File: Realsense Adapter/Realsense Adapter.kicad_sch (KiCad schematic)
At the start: 2 parts, among them J1 USB3_B_Micro

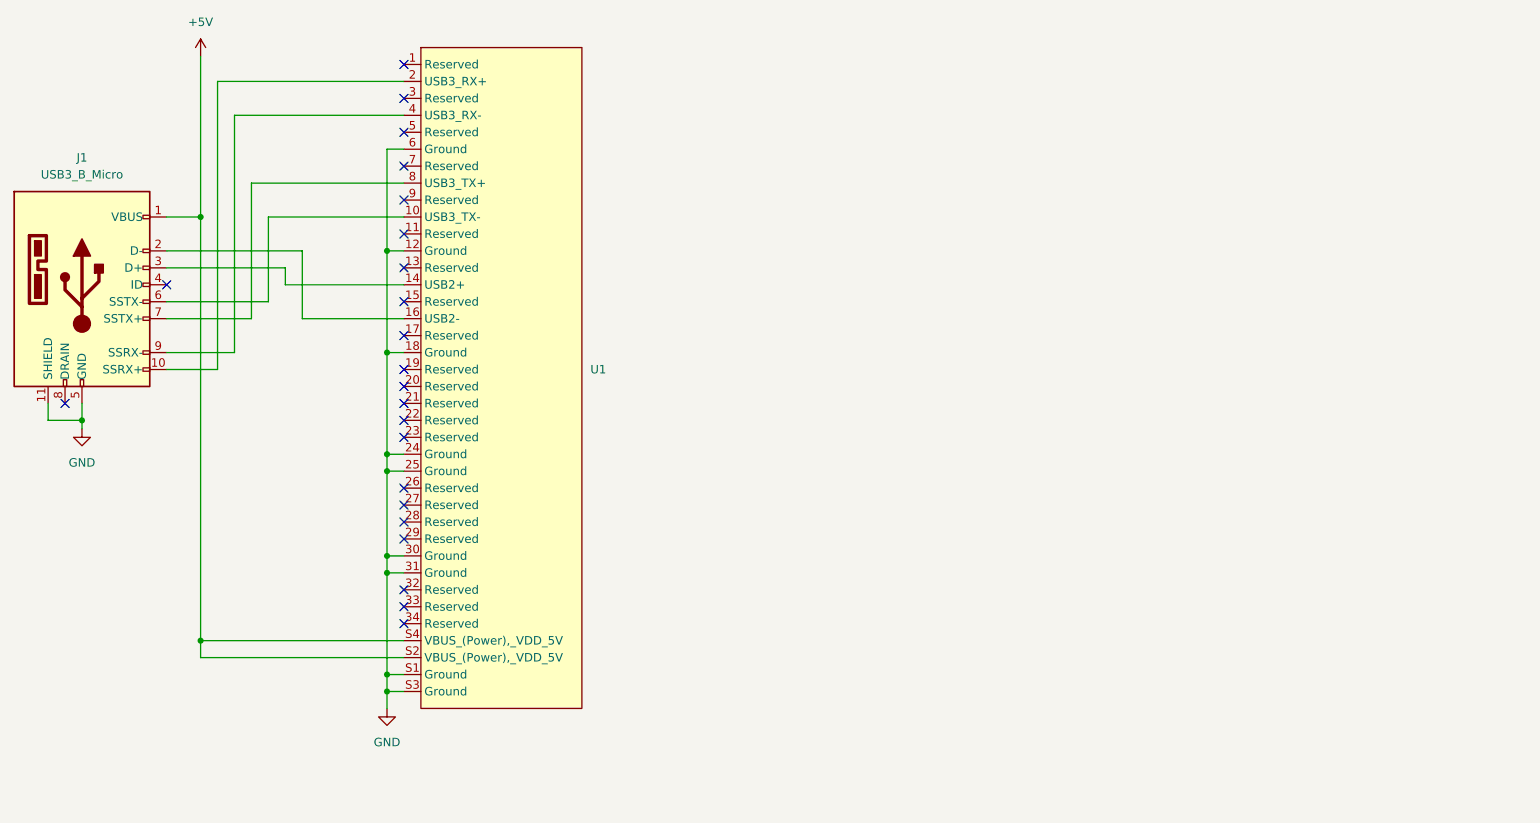
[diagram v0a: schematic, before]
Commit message: Version v1.0-PROTO of Realsense adapter complete
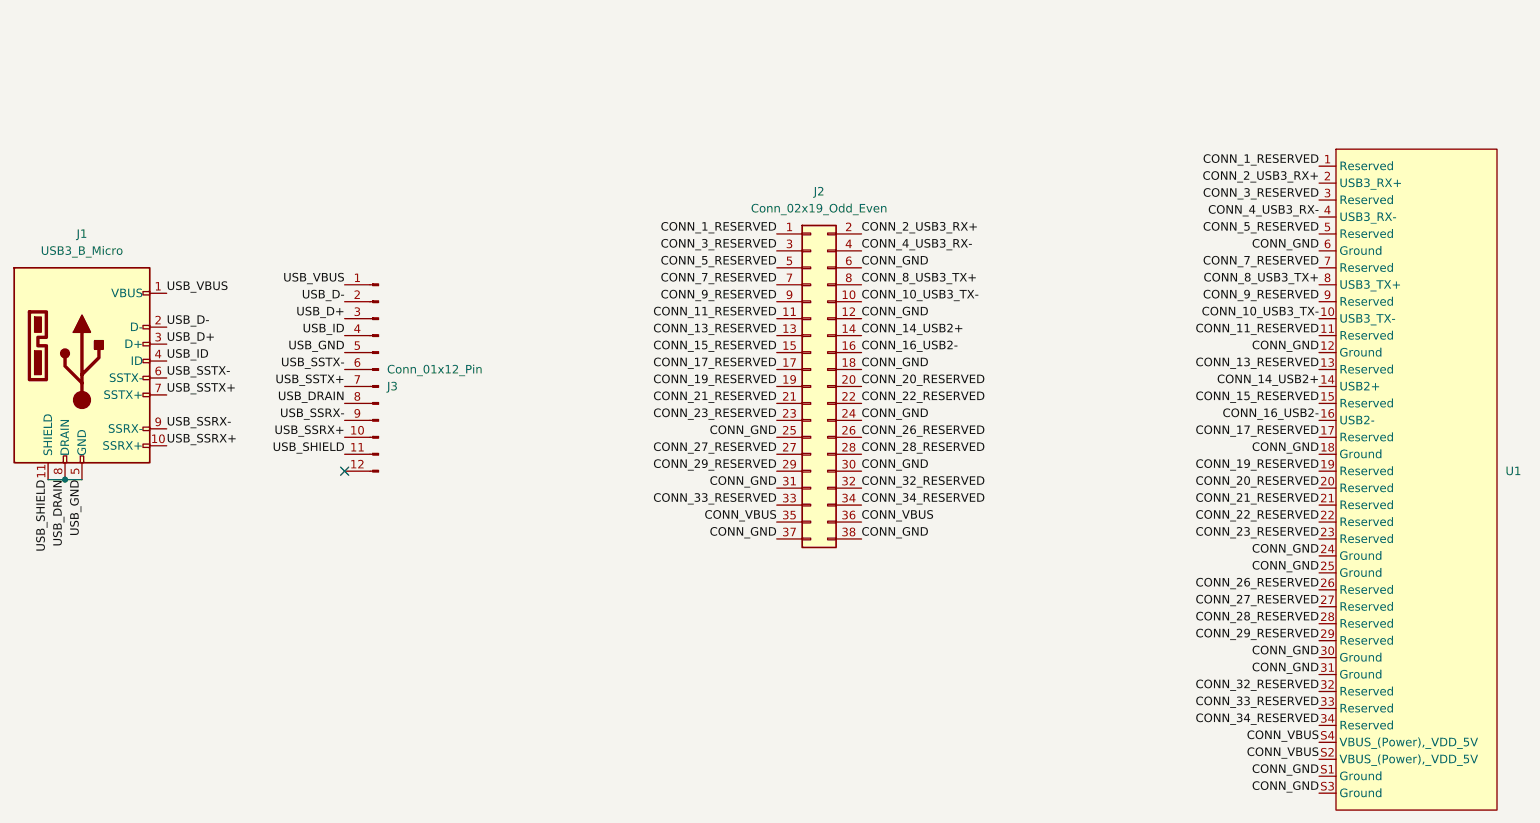
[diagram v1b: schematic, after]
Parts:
- added J2: Conn_02x19_Odd_Even, Connector_PinHeader_2.54mm:PinHeader_2x19_P2.54mm_Vertical, symbol Connector_Generic:Conn_02x19_Odd_Even
- added J3: Conn_01x12_Pin, Connector_PinHeader_2.54mm:PinHeader_1x12_P2.54mm_Vertical, symbol Connector:Conn_01x12_Pin
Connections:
- net CONN_2_USB3_RX+: now reaches U1.2 (USB3_RX+)
- net CONN_2_USB3_RX+: now also J2.2 (Pin_2); no longer J1.10 (SSRX+)
- net CONN_16_USB2-: now reaches U1.16 (USB2-)
- net CONN_16_USB2-: now also J2.16 (Pin_16); no longer J1.2 (D-)
- net CONN_14_USB2+: now reaches U1.14 (USB2+)
- net CONN_14_USB2+: now also J2.14 (Pin_14); no longer J1.3 (D+)
- net USB_ID: now reaches J1.4 (ID)
- net USB_ID: now also J3.4 (Pin_4)
- net CONN_10_USB3_TX-: now reaches U1.10 (USB3_TX-)
- net CONN_10_USB3_TX-: now also J2.10 (Pin_10); no longer J1.6 (SSTX-)
- net CONN_8_USB3_TX+: now reaches U1.8 (USB3_TX+)
- net CONN_8_USB3_TX+: now also J2.8 (Pin_8); no longer J1.7 (SSTX+)
- net USB_DRAIN: now reaches J1.8 (DRAIN)
- net USB_DRAIN: now also J1.11 (SHIELD), J1.5 (GND), J3.11 (Pin_11), J3.5 (Pin_5), J3.8 (Pin_8)
- net CONN_4_USB3_RX-: now reaches U1.4 (USB3_RX-)
- net CONN_4_USB3_RX-: now also J2.4 (Pin_4); no longer J1.9 (SSRX-)
- net CONN_1_RESERVED: now reaches U1.1 (Reserved)
- net CONN_1_RESERVED: now also J2.1 (Pin_1)
- net CONN_11_RESERVED: now reaches U1.11 (Reserved)
- net CONN_11_RESERVED: now also J2.11 (Pin_11)
- net CONN_13_RESERVED: now reaches U1.13 (Reserved)
- net CONN_13_RESERVED: now also J2.13 (Pin_13)
- net CONN_15_RESERVED: now reaches U1.15 (Reserved)
- net CONN_15_RESERVED: now also J2.15 (Pin_15)
- net CONN_17_RESERVED: now reaches U1.17 (Reserved)
- net CONN_17_RESERVED: now also J2.17 (Pin_17)
- net CONN_19_RESERVED: now reaches U1.19 (Reserved)
- net CONN_19_RESERVED: now also J2.19 (Pin_19)
- net CONN_20_RESERVED: now reaches U1.20 (Reserved)
- net CONN_20_RESERVED: now also J2.20 (Pin_20)
- net CONN_21_RESERVED: now reaches U1.21 (Reserved)
- net CONN_21_RESERVED: now also J2.21 (Pin_21)
- net CONN_22_RESERVED: now reaches U1.22 (Reserved)
- net CONN_22_RESERVED: now also J2.22 (Pin_22)
- net CONN_23_RESERVED: now reaches U1.23 (Reserved)
- net CONN_23_RESERVED: now also J2.23 (Pin_23)
- net CONN_26_RESERVED: now reaches U1.26 (Reserved)
- net CONN_26_RESERVED: now also J2.26 (Pin_26)
- net CONN_27_RESERVED: now reaches U1.27 (Reserved)
- net CONN_27_RESERVED: now also J2.27 (Pin_27)
- net CONN_28_RESERVED: now reaches U1.28 (Reserved)
- net CONN_28_RESERVED: now also J2.28 (Pin_28)
- net CONN_29_RESERVED: now reaches U1.29 (Reserved)
- net CONN_29_RESERVED: now also J2.29 (Pin_29)
- net CONN_3_RESERVED: now reaches U1.3 (Reserved)
- net CONN_3_RESERVED: now also J2.3 (Pin_3)
- net CONN_32_RESERVED: now reaches U1.32 (Reserved)
- net CONN_32_RESERVED: now also J2.32 (Pin_32)
- net CONN_33_RESERVED: now reaches U1.33 (Reserved)
- net CONN_33_RESERVED: now also J2.33 (Pin_33)
- net CONN_34_RESERVED: now reaches U1.34 (Reserved)
- net CONN_34_RESERVED: now also J2.34 (Pin_34)
- net CONN_5_RESERVED: now reaches U1.5 (Reserved)
- net CONN_5_RESERVED: now also J2.5 (Pin_5)
- net CONN_7_RESERVED: now reaches U1.7 (Reserved)
- net CONN_7_RESERVED: now also J2.7 (Pin_7)
- net CONN_9_RESERVED: now reaches U1.9 (Reserved)
- net CONN_9_RESERVED: now also J2.9 (Pin_9)
- net +5V renamed CONN_VBUS
- net CONN_VBUS: now also J2.35 (Pin_35), J2.36 (Pin_36); no longer J1.1 (VBUS)
- net GND renamed CONN_GND
- net CONN_GND: now also J2.12 (Pin_12), J2.18 (Pin_18), J2.24 (Pin_24), J2.25 (Pin_25), J2.30 (Pin_30), J2.31 (Pin_31), J2.37 (Pin_37), J2.38 (Pin_38), J2.6 (Pin_6); no longer J1.11 (SHIELD), J1.5 (GND)
- new net USB_D+: J1.3 (D+), J3.3 (Pin_3)
- new net USB_D-: J1.2 (D-), J3.2 (Pin_2)
- new net USB_SSRX+: J1.10 (SSRX+), J3.10 (Pin_10)
- new net USB_SSRX-: J1.9 (SSRX-), J3.9 (Pin_9)
- new net USB_SSTX+: J1.7 (SSTX+), J3.7 (Pin_7)
- new net USB_SSTX-: J1.6 (SSTX-), J3.6 (Pin_6)
- new net USB_VBUS: J1.1 (VBUS), J3.1 (Pin_1)
- no-connect marks 23 -> 1
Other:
- company: (none) -> Utah Student Robotics
- title: (none) -> Intel Realsense Breakout Board
- moved on the sheet: J1, U1
